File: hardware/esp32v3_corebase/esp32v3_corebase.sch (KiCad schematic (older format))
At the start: 38 parts, among them J1 USB_C_Receptacle_USB2.0, Q1 MBT2222ADW1T1, U1 TLV75533PDBV, U3 W25Q32FVSS, U4 CH340C, U5 ESP32, Y1 40MHz 10ppm

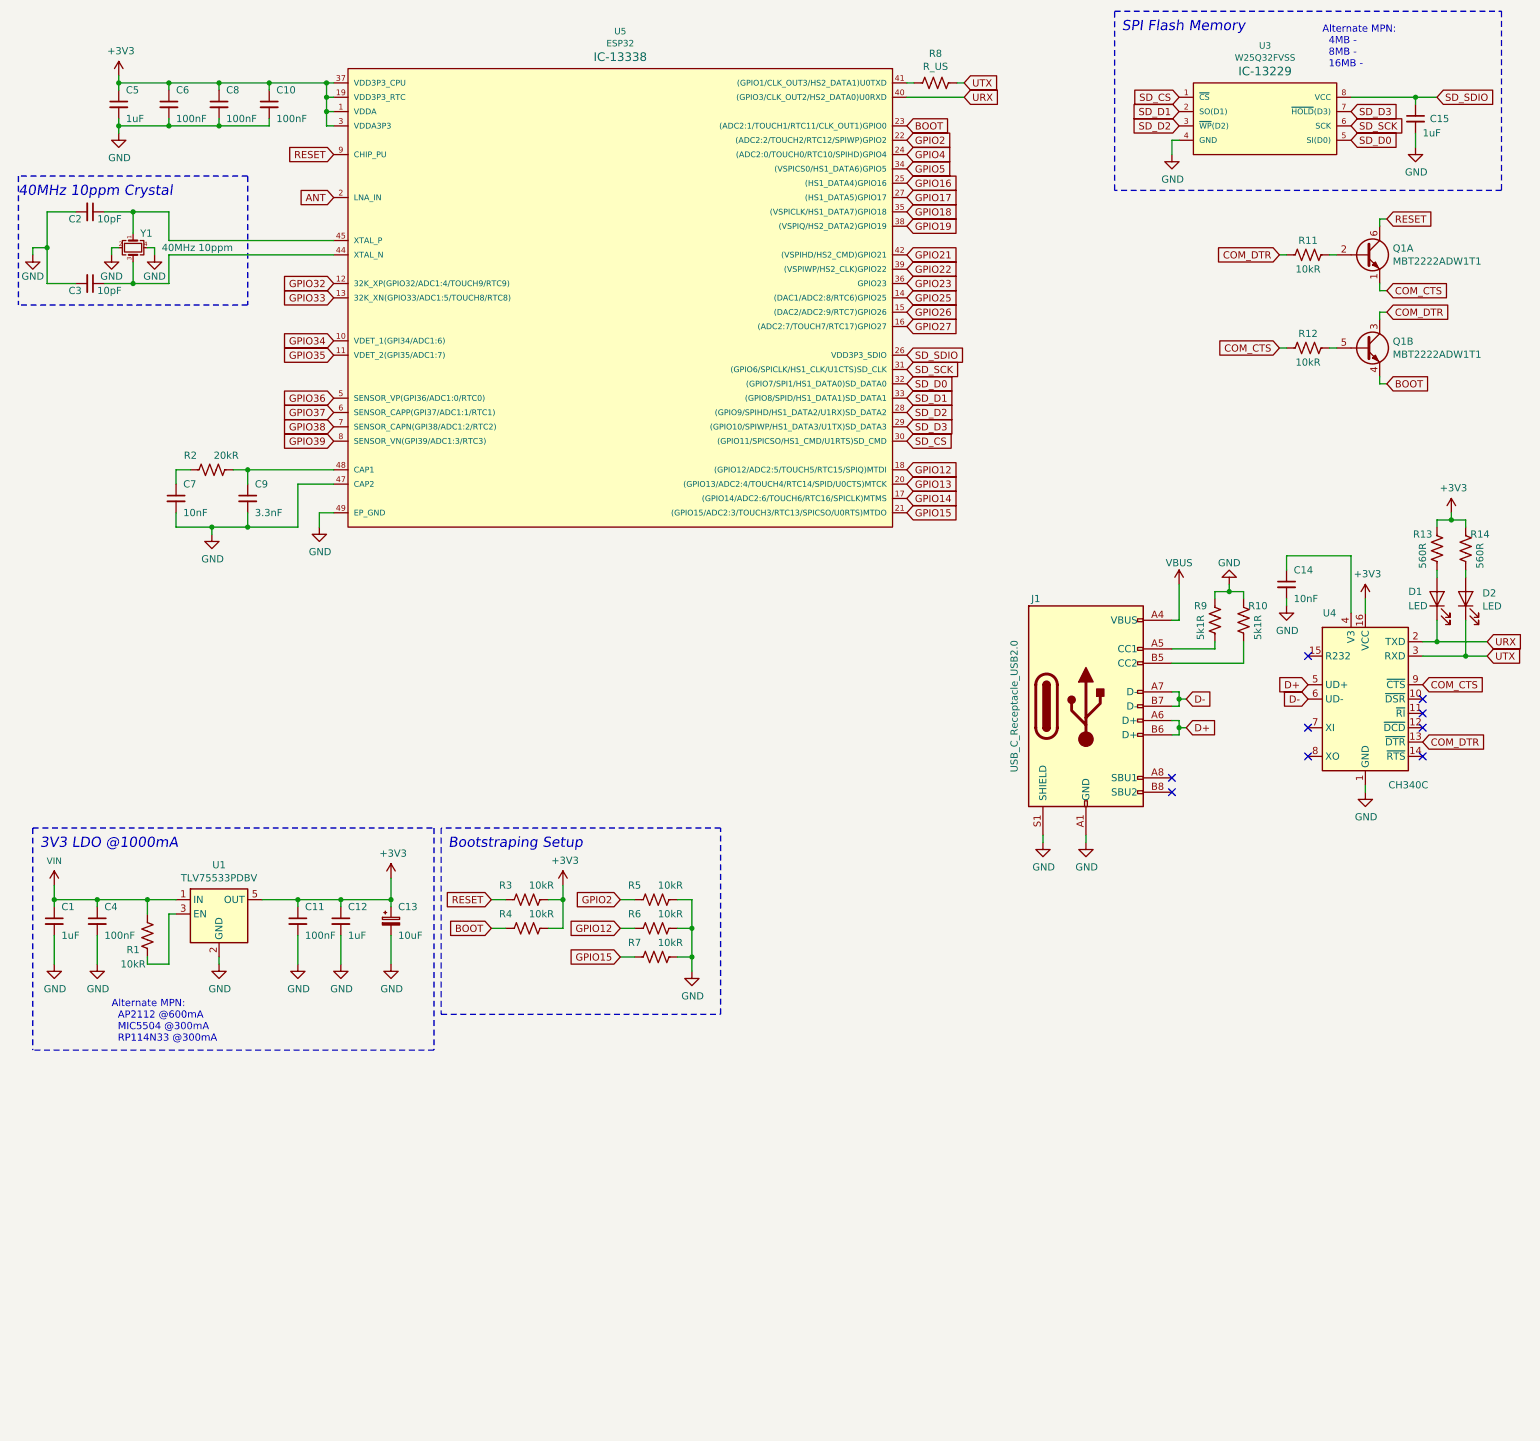
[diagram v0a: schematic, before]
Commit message: [FEATURE] Minor changes on the circuit and VIN to 5V
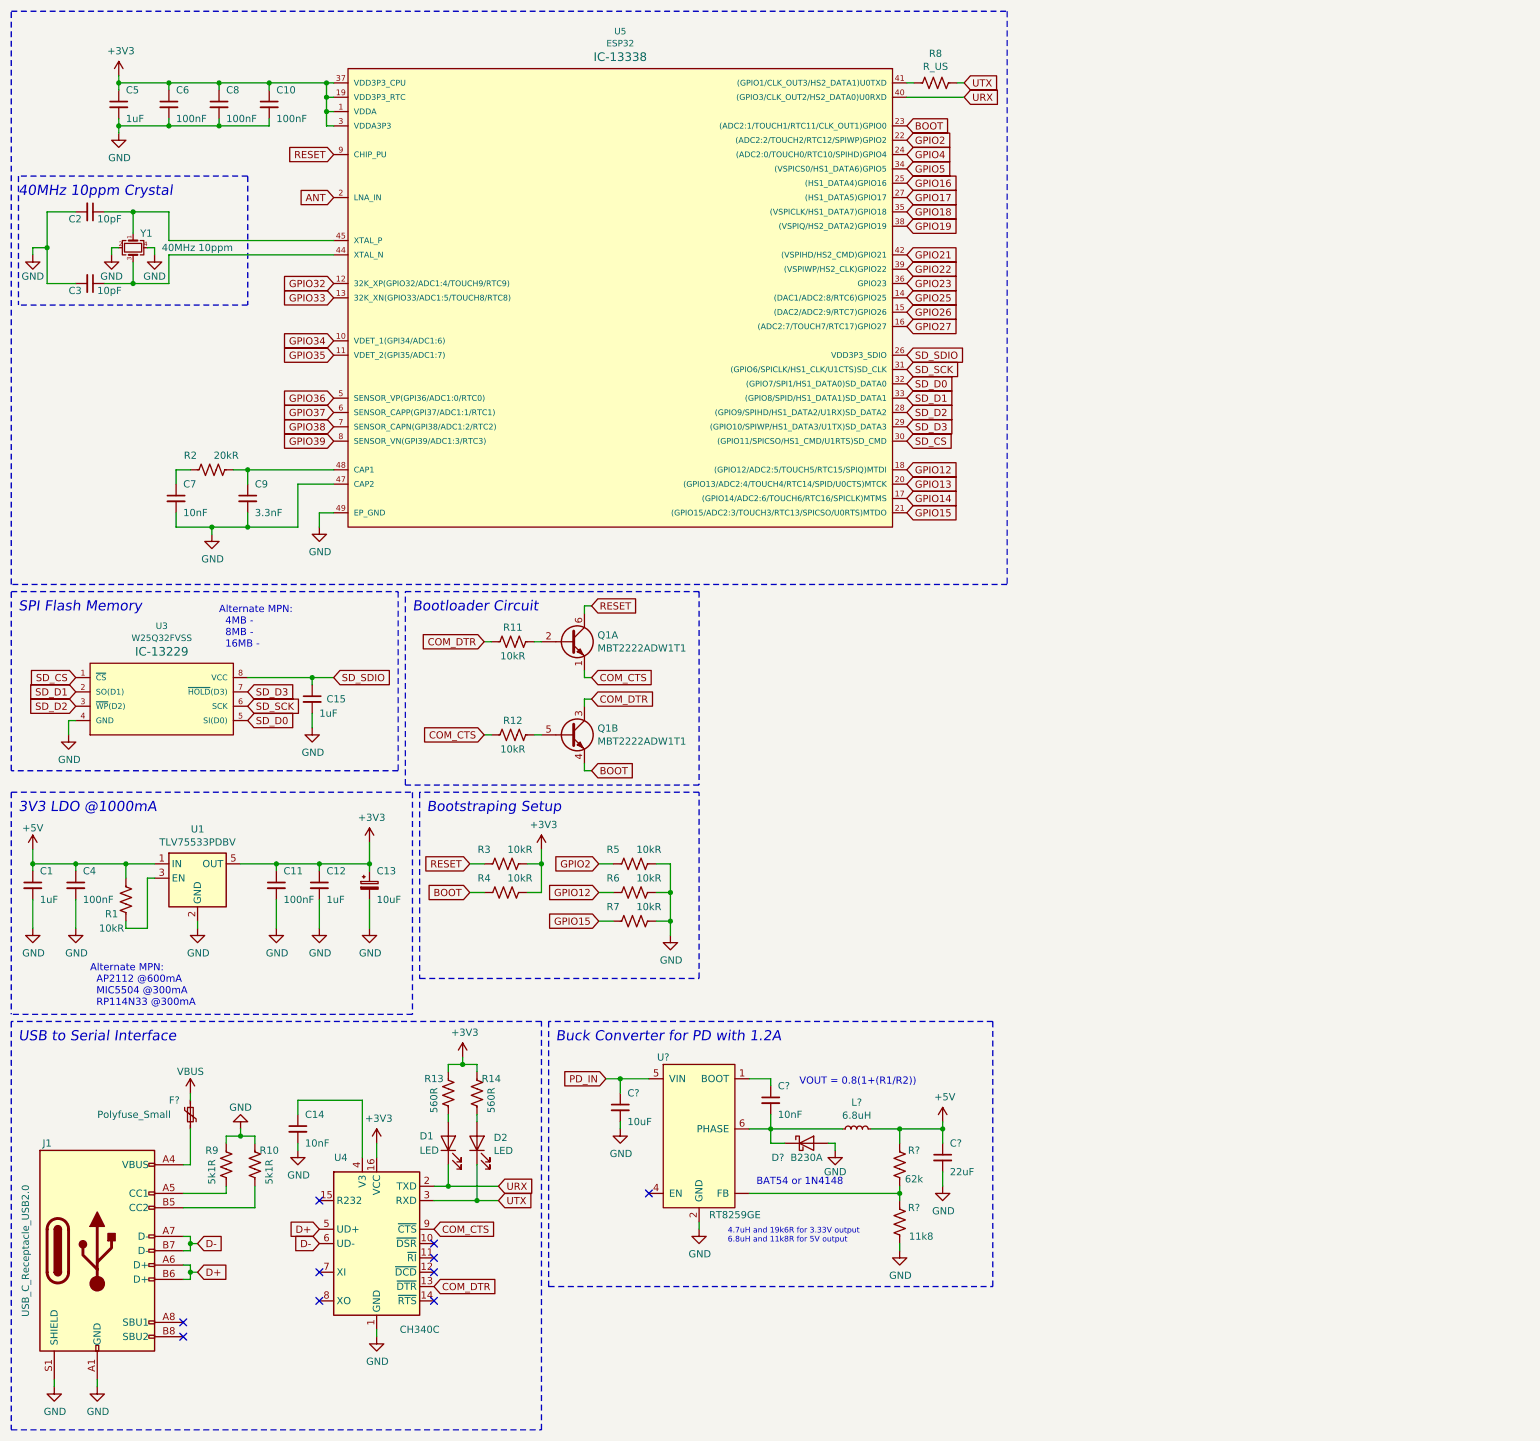
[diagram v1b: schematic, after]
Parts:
- added C?: 10uF, Capacitor_SMD:C_0402_1005Metric, symbol Device:C_Small
- added C?: 10nF, Capacitor_SMD:C_0402_1005Metric, symbol Device:C_Small
- added C?: 22uF, Capacitor_SMD:C_0402_1005Metric, symbol Device:C_Small
- added D?: B230A, symbol Device:D_Schottky
- added F?: Polyfuse_Small, symbol Device:Polyfuse_Small
- added L?: 6.8uH, symbol Device:L_Small
- added R?: 62k, Resistor_SMD:R_0402_1005Metric, symbol Device:R_US
- added R?: 11k8, Resistor_SMD:R_0402_1005Metric, symbol Device:R_US
- added U?: RT8259GE, Package_TO_SOT_SMD:SOT-23-6, symbol Buck_Regulators:RT8259GE
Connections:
- net GND: now also C?.2, C?.2, D?.2 (A), R?.1, U?.2 (GND)
- net VBUS: now also F?.1; no longer J1.A4 (VBUS), J1.A9 (VBUS), J1.B4 (VBUS), J1.B9 (VBUS)
- net VIN renamed +5V
- net +5V: now also C?.1, L?.2, R?.2
- new net: F?.2, J1.A4 (VBUS), J1.A9 (VBUS), J1.B4 (VBUS), J1.B9 (VBUS)
- new net: C?.1, U?.1 (BOOT)
- new net: C?.2, D?.1 (K), L?.1, U?.6 (PHASE)
- new net: R?.1, R?.2, U?.~ (FB)
- new net PD_IN: C?.1, U?.5 (VIN)
- no-connect marks 9 -> 10
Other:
- note added: "4.7uH and 19k6R for 3.33V output\n6.8uH and 11k8R for 5V output"
- note added: "BAT54 or 1N4148"
- note added: "Bootloader Circuit"
- note added: "Buck Converter for PD with 1.2A"
- note added: "USB to Serial Interface"
- note added: "VOUT = 0.8(1+(R1/R2))"
- moved on the sheet: C1, C11, C12, C13, C14, C15, C4, D1, D2, J1, Q1A, Q1B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
